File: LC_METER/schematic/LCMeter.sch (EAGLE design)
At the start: 207 parts, among them IC1 MEGA8535, IC10 MC34063, IC2 74HC595, IC3 74HC595, IC4 74HC595, IC5 74HC595, IC6 74HC595, IC7 LM324, IC8 7905, IC9 LM317, J10 0, J100 0, J4 0, J6 0, J8 0, Q1 12MHz, T1 BC847, T2 BC857, T3 BC847, T4 BC847, T5 BC847, T6 BC847, T7 BC857, X1 MCU_PROGRAMMING, X2 L_X, X3 C_X, X4 USB_MICRO, X5 USB_B

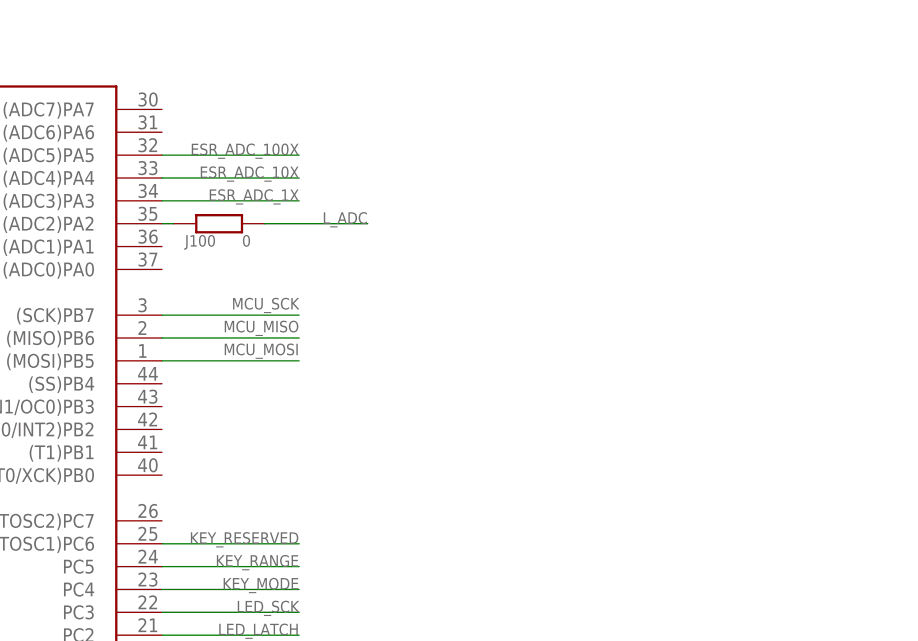
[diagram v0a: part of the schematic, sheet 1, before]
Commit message: LCMeter start routing4
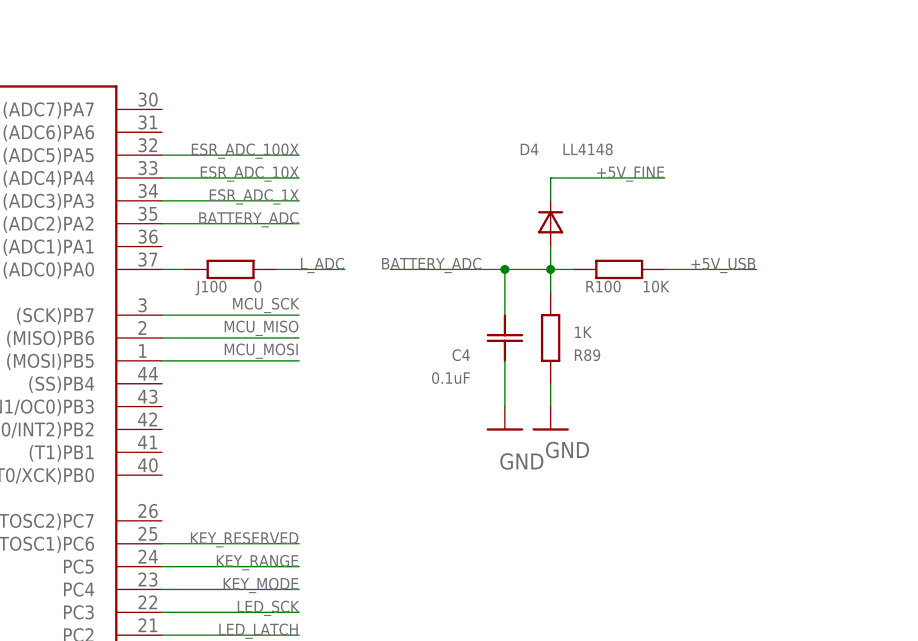
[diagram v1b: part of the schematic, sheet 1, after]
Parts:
- added C4: 0.1uF, __MyCommonLib1:CSMD_0805
- added D4: LL4148, __MyCommonLib1:LL4147SOD-80
- added J11: 0, __MyCommonLib1:RSMD_0805
- added R100: 10K, __MyCommonLib1:RSMD_0805
- added R89: 1K, __MyCommonLib1:RSMD_0805
- D28: device __MyCommonLib1:1N4001DO-41_10MM -> __MyCommonLib1:1N4001DO-41_5MM
- R59: device __MyCommonLib1:RSMD_0805 -> __MyCommonLib1:RSMD_1206_BIG_GAP
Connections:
- new net BATTERY_ADC: C4.PIN1, D4.ANODE, IC1.(ADC2)PA2, R100.PIN1, R89.PIN0
- new net N$101: J11.PIN0, X4.D-
- net +5V_FINE: now also D4.CATHODE
- net +5V_USB: now also R100.PIN0
- net GND: now also C4.PIN0, R89.PIN1
- net N$100: now also IC1.(ADC0)PA0; no longer IC1.(ADC2)PA2
- net USB_D-: now also J11.PIN1; no longer X4.D-
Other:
- moved on the sheet: J100
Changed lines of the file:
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@@
 <part name="R54" library="__MyCommonLib1" deviceset="R" device="SMD_0805" value="100K"/>
 <part name="GND12" library="supply1" deviceset="GND" device=""/>
-<part name="R59" library="__MyCommonLib1" deviceset="R" device="SMD_0805" value="300R"/>
+<part name="R59" library="__MyCommonLib1" deviceset="R" device="SMD_1206_BIG_GAP" value="300R"/>
 <part name="D10" library="__MyCommonLib1" deviceset="LL4147" device="SOD-80" value="LL4148"/>
 <part name="C20" library="__MyCommonLib1" deviceset="C" device="SMD_0805" value="0.1uF"/>
@@
 <part name="GND71" library="supply1" deviceset="GND" device=""/>
 <part name="GND72" library="supply1" deviceset="GND" device=""/>
-<part name="D28" library="__MyCommonLib1" deviceset="1N4001" device="DO-41_10MM" value="FR207"/>
+<part name="D28" library="__MyCommonLib1" deviceset="1N4001" device="DO-41_5MM" value="FR207"/>
 <part name="D29" library="__MyCommonLib1" deviceset="1N4001" device="DO-41_5MM" value="FR207"/>
 <part name="C56" library="__MyCommonLib1" deviceset="C" device="SMD_1206_BIG_GAP" value="0.47uFx16V"/>
@@
 <part name="GND81" library="supply1" deviceset="GND" device=""/>
 <part name="GND86" library="supply1" deviceset="GND" device=""/>
+<part name="J11" library="__MyCommonLib1" deviceset="R" device="SMD_0805" value="0"/>
+<part name="R100" library="__MyCommonLib1" deviceset="R" device="SMD_0805" value="10K"/>
+<part name="R89" library="__MyCommonLib1" deviceset="R" device="SMD_0805" value="1K"/>
+<part name="C4" library="__MyCommonLib1" deviceset="C" device="SMD_0805" value="0.1uF"/>
+<part name="D4" library="__MyCommonLib1" deviceset="LL4147" device="SOD-80" value="LL4148"/>
+<part name="GND43" library="supply1" deviceset="GND" device=""/>
+<part name="GND88" library="supply1" deviceset="GND" device=""/>
 </parts>
 <sheets>
@@
 <attribute name="VALUE" x="196.85" y="102.87" size="1.778" layer="96" font="vector" ratio="20"/>
 </instance>
-<instance part="J100" gate="R$1" x="95.25" y="149.86" smashed="yes" rot="R90">
-<attribute name="NAME" x="91.44" y="147.32" size="1.27" layer="95" font="vector" ratio="20"/>
-<attribute name="VALUE" x="97.79" y="147.32" size="1.27" layer="96" font="vector" ratio="20"/>
+<instance part="J100" gate="R$1" x="96.52" y="144.78" smashed="yes" rot="R90">
+<attribute name="NAME" x="92.71" y="142.24" size="1.27" layer="95" font="vector" ratio="20"/>
+<attribute name="VALUE" x="99.06" y="142.24" size="1.27" layer="96" font="vector" ratio="20"/>
+</instance>
+<instance part="R100" gate="R$1" x="139.7" y="144.78" smashed="yes" rot="R90">
+<attribute name="NAME" x="135.89" y="142.24" size="1.27" layer="95" font="vector" ratio="20"/>
+<attribute name="VALUE" x="142.24" y="142.24" size="1.27" layer="96" font="vector" ratio="20"/>
+</instance>
+<instance part="R89" gate="R$1" x="132.08" y="137.16" smashed="yes" rot="R180">
+<attribute name="NAME" x="134.62" y="134.62" size="1.27" layer="95" font="vector" ratio="20"/>
+<attribute name="VALUE" x="134.62" y="137.16" size="1.27" layer="96" font="vector" ratio="20"/>
+</instance>
+<instance part="C4" gate="C$1" x="127" y="137.16" smashed="yes" rot="MR0">
+<attribute name="NAME" x="123.19" y="134.62" size="1.27" layer="95" font="vector" ratio="20" rot="MR0"/>
+<attribute name="VALUE" x="123.19" y="132.08" size="1.27" layer="96" font="vector" ratio="20" rot="MR0"/>
+</instance>
+<instance part="D4" gate="D1" x="132.08" y="149.86" smashed="yes">
+<attribute name="NAME" x="130.81" y="158.75" size="1.27" layer="95" font="vector" ratio="20" rot="R180"/>
+<attribute name="VALUE" x="133.35" y="157.48" size="1.27" layer="96" font="vector" ratio="20"/>
+</instance>
+<instance part="GND43" gate="1" x="132.08" y="127" smashed="yes">
+<attribute name="VALUE" x="131.445" y="123.825" size="1.778" layer="96" font="vector" ratio="20"/>
+</instance>
+<instance part="GND88" gate="1" x="127" y="127" smashed="yes">
+<attribute name="VALUE" x="126.365" y="122.555" size="1.778" layer="96" font="vector" ratio="20"/>
 </instance>
 </instances>
@@
 <pinref part="GND98" gate="1" pin="GND"/>
 </segment>
+<segment>
+<pinref part="C4" gate="C$1" pin="PIN0"/>
+<pinref part="GND88" gate="1" pin="GND"/>
+<wire x1="127" y1="134.62" x2="127" y2="129.54" width="0.1524" layer="91"/>
+</segment>
+<segment>
+<pinref part="R89" gate="R$1" pin="PIN1"/>
+<pinref part="GND43" gate="1" pin="GND"/>
+<wire x1="132.08" y1="132.08" x2="132.08" y2="129.54" width="0.1524" layer="91"/>
+</segment>
 </net>
 <net name="USB_D-" class="0">
@@
 <label x="208.28" y="113.665" size="1.27" layer="95" font="vector" ratio="20" rot="R180"/>
 </segment>
+<segment>
+<pinref part="D4" gate="D1" pin="CATHODE"/>
+<wire x1="132.08" y1="152.4" x2="132.08" y2="154.94" width="0.1524" layer="91"/>
+<wire x1="132.08" y1="154.94" x2="144.78" y2="154.94" width="0.1524" layer="91"/>
+<label x="144.78" y="156.21" size="1.27" layer="95" font="vector" ratio="20" rot="R180"/>
+</segment>
 </net>
 <net name="N$141" class="0">
@@
 <net name="L_ADC" class="0">
 <segment>
-<wire x1="100.33" y1="149.86" x2="111.76" y2="149.86" width="0.1524" layer="91"/>
-<label x="111.76" y="151.13" size="1.27" layer="95" font="vector" ratio="20" rot="R180"/>
+<wire x1="101.6" y1="144.78" x2="109.22" y2="144.78" width="0.1524" layer="91"/>
+<label x="109.22" y="146.05" size="1.27" layer="95" font="vector" ratio="20" rot="R180"/>
 <pinref part="J100" gate="R$1" pin="PIN0"/>
 </segment>
@@
 </segment>
 </net>
-<net name="N$100" class="0">
+<net name="BATTERY_ADC" class="0">
+<segment>
+<pinref part="C4" gate="C$1" pin="PIN1"/>
+<pinref part="R100" gate="R$1" pin="PIN1"/>
+<wire x1="127" y1="139.7" x2="127" y2="144.78" width="0.1524" layer="91"/>
+<wire x1="127" y1="144.78" x2="132.08" y2="144.78" width="0.1524" layer="91"/>
+<pinref part="R89" gate="R$1" pin="PIN0"/>
+<wire x1="132.08" y1="144.78" x2="134.62" y2="144.78" width="0.1524" layer="91"/>
+<wire x1="132.08" y1="142.24" x2="132.08" y2="144.78" width="0.1524" layer="91"/>
+<pinref part="D4" gate="D1" pin="ANODE"/>
+<wire x1="132.08" y1="147.32" x2="132.08" y2="144.78" width="0.1524" layer="91"/>
+<wire x1="114.3" y1="144.78" x2="127" y2="144.78" width="0.1524" layer="91"/>
+<junction x="127" y="144.78"/>
+<junction x="132.08" y="144.78"/>
+<label x="124.46" y="146.05" size="1.27" layer="95" font="vector" ratio="20" rot="R180"/>
+</segment>
 <segment>
 <pinref part="IC1" gate="G$1" pin="(ADC2)PA2"/>
+<wire x1="88.9" y1="149.86" x2="104.14" y2="149.86" width="0.1524" layer="91"/>
+<label x="104.14" y="151.13" size="1.27" layer="95" font="vector" ratio="20" rot="R180"/>
+</segment>
+</net>
+<net name="+5V_USB" class="0">
+<segment>
+<pinref part="R100" gate="R$1" pin="PIN0"/>
+<wire x1="144.78" y1="144.78" x2="154.94" y2="144.78" width="0.1524" layer="91"/>
+<label x="154.94" y="146.05" size="1.27" layer="95" font="vector" ratio="20" rot="R180"/>
+</segment>
+</net>
+<net name="N$100" class="0">
+<segment>
+<pinref part="IC1" gate="G$1" pin="(ADC0)PA0"/>
 <pinref part="J100" gate="R$1" pin="PIN1"/>
-<wire x1="90.17" y1="149.86" x2="88.9" y2="149.86" width="0.1524" layer="91"/>
+<wire x1="88.9" y1="144.78" x2="91.44" y2="144.78" width="0.1524" layer="91"/>
 </segment>
 </net>
@@
 <attribute name="VALUE" x="200.66" y="146.685" size="1.27" layer="96" font="vector" ratio="20" rot="MR180"/>
 </instance>
+<instance part="J11" gate="R$1" x="38.1" y="154.94" smashed="yes" rot="R270">
+<attribute name="NAME" x="35.56" y="156.21" size="1.27" layer="95" font="vector" ratio="20"/>
+<attribute name="VALUE" x="41.91" y="157.48" size="1.27" layer="96" font="vector" ratio="20" rot="R180"/>
+</instance>
 </instances>
 <busses>
@@
 <junction x="45.72" y="129.54"/>
 <label x="53.34" y="131.445" size="1.27" layer="95" font="vector" ratio="20" rot="R180"/>
+<wire x1="43.18" y1="154.94" x2="45.72" y2="154.94" width="0.1524" layer="91"/>
 <wire x1="45.72" y1="154.94" x2="45.72" y2="129.54" width="0.1524" layer="91"/>
-<pinref part="X4" gate="X$1" pin="D-"/>
-<wire x1="25.4" y1="154.94" x2="45.72" y2="154.94" width="0.1524" layer="91"/>
+<pinref part="J11" gate="R$1" pin="PIN1"/>
 </segment>
 </net>
@@
 </segment>
 </net>
+<net name="N$101" class="0">
+<segment>
+<pinref part="X4" gate="X$1" pin="D-"/>
+<pinref part="J11" gate="R$1" pin="PIN0"/>
+<wire x1="33.02" y1="154.94" x2="25.4" y2="154.94" width="0.1524" layer="91"/>
+</segment>
+</net>
